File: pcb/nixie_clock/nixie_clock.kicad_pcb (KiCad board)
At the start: 6 copper layers, 218.5 x 53.2 mm, 175 parts, among them J1 Conn_01x06_Pin, Q1 Q_NMOS_GDS, T1 750312367, U1 MSD42WT1G, U10 MSD42WT1G, U11 MSD42WT1G, U12 MSD42WT1G, U13 PCA9685BS, U14 PicoW, U15 PCA9685BS, U16 MSD42WT1G, U17 MSD42WT1G, U18 MSD42WT1G, U19 MSD42WT1G, U2 MSD42WT1G, U20 MSD42WT1G, U21 MSD42WT1G, U22 MSD42WT1G, U23 MSD42WT1G, U24 MSD42WT1G, U25 MSD42WT1G, U26 MSD42WT1G, U27 MSD42WT1G, U28 PCA9685BS, U29 MSD42WT1G, U3 MSD42WT1G, U30 MSD42WT1G, U31 MSD42WT1G, U32 MSD42WT1G, U33 MSD42WT1G, U34 MSD42WT1G, U35 MSD42WT1G, U36 MSD42WT1G, U37 MSD42WT1G, U38 MSD42WT1G, U39 MSD42WT1G, U4 MSD42WT1G, U40 MSD42WT1G, U41 PCA9685BS, U42 MSD42WT1G, U43 MSD42WT1G, U44 MSD42WT1G, U45 MSD42WT1G, U46 MSD42WT1G, U47 MSD42WT1G, U48 MSD42WT1G, U49 MSD42WT1G, U5 MSD42WT1G, U50 MSD42WT1G, U51 MSD42WT1G, U52 MSD42WT1G, U53 MSD42WT1G, U54 PCA9685BS, U55 MSD42WT1G, U56 MSD42WT1G, U57 MSD42WT1G, U58 MSD42WT1G, U59 MSD42WT1G, U6 MSD42WT1G, U60 MSD42WT1G, U61 MSD42WT1G, U62 MSD42WT1G, U63 MSD42WT1G, U64 MSD42WT1G, U65 MSD42WT1G, U66 MSD42WT1G, U67 MSD42WT1G, U68 MSD42WT1G, U69 MSD42WT1G, U7 MSD42WT1G, U70 MSD42WT1G, U71 MSD42WT1G, U72 MSD42WT1G, U73 MSD42WT1G, U74 MSD42WT1G, U75 MSD42WT1G, U76 MSD42WT1G, U77 MSD42WT1G, U78 MSD42WT1G, U79 LT3759EMSE#TRPBF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

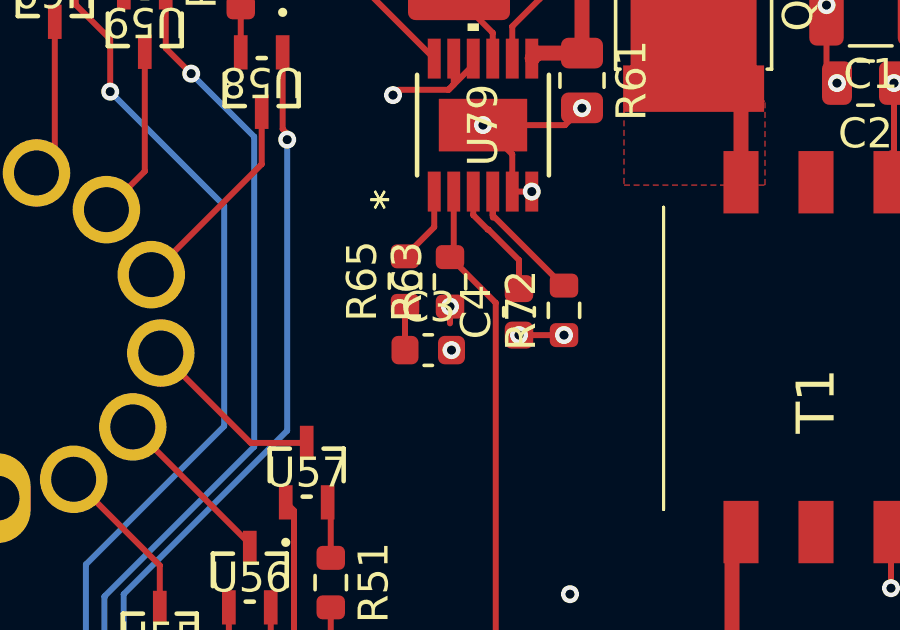
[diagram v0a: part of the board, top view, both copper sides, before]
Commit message: changes and improvements
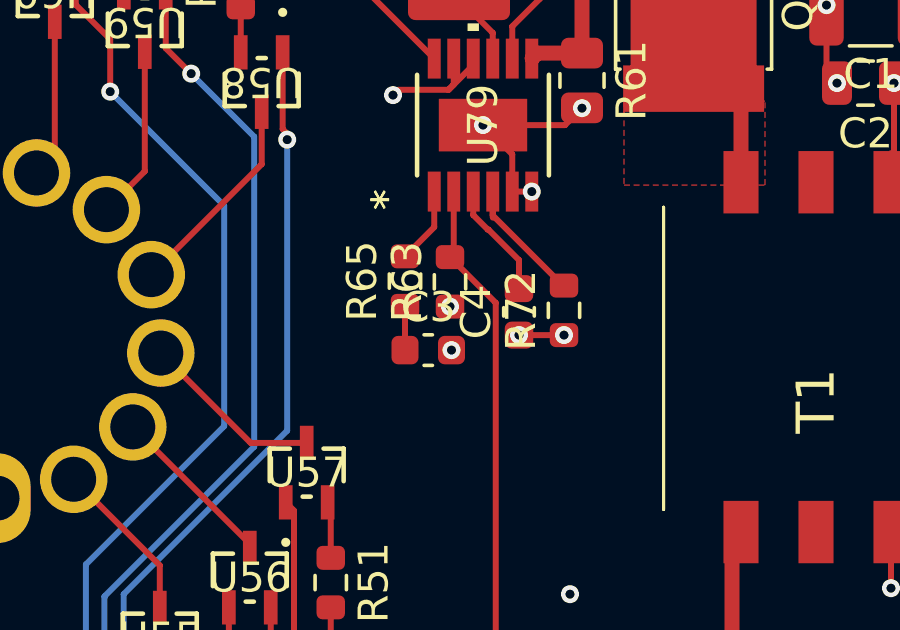
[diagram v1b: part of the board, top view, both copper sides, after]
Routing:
- net GND: track 235.4 -> 234.8 mm
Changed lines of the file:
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@@
 	(dimension
 		(type aligned)
-		(layer "F.Cu")
+		(layer "User.1")
 		(pts
 			(xy 45.6 77.6) (xy 264.15 77.6)
@@
 		(gr_text "218.5500 mm"
 			(at 154.875 69.4 0)
-			(layer "F.Cu")
+			(layer "User.1")
 			(effects
 				(font
@@
 	(dimension
 		(type aligned)
-		(layer "F.Cu")
+		(layer "User.1")
 		(pts
 			(xy 264.15 77.6) (xy 264.15 130.85)
@@
 		(gr_text "53.2500 mm"
 			(at 274.8 104.225 90)
-			(layer "F.Cu")
+			(layer "User.1")
 			(effects
 				(font
@@
 		(width 0.2)
 		(layer "F.Cu")
-		(net 1)
-	)
-	(segment
-		(start 239.5 99.475)
-		(end 239.5 98.915)
-		(width 0.2)
-		(layer "F.Cu")
